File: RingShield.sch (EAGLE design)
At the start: 37 parts, among them U1 LED-ADDRESSABLE16MM, U10 LED-ADDRESSABLE16MM, U11 LED-ADDRESSABLE16MM, U12 LED-ADDRESSABLE16MM, U13 LED-ADDRESSABLE16MM, U14 LED-ADDRESSABLE16MM, U15 LED-ADDRESSABLE16MM, U16 LED-ADDRESSABLE16MM, U17 LED-ADDRESSABLE16MM, U18 LED-ADDRESSABLE16MM, U19 LED-ADDRESSABLE16MM, U2 LED-ADDRESSABLE16MM, U20 LED-ADDRESSABLE16MM, U21 LED-ADDRESSABLE16MM, U22 LED-ADDRESSABLE16MM, U23 LED-ADDRESSABLE16MM, U24 LED-ADDRESSABLE16MM, U25 LED-ADDRESSABLE16MM, U26 LED-ADDRESSABLE16MM, U27 LED-ADDRESSABLE16MM, U28 LED-ADDRESSABLE16MM, U29 LED-ADDRESSABLE16MM, U3 LED-ADDRESSABLE16MM, U30 LED-ADDRESSABLE16MM, U4 LED-ADDRESSABLE16MM, U5 LED-ADDRESSABLE16MM, U6 LED-ADDRESSABLE16MM, U7 LED-ADDRESSABLE16MM, U8 LED-ADDRESSABLE16MM, U9 LED-ADDRESSABLE16MM

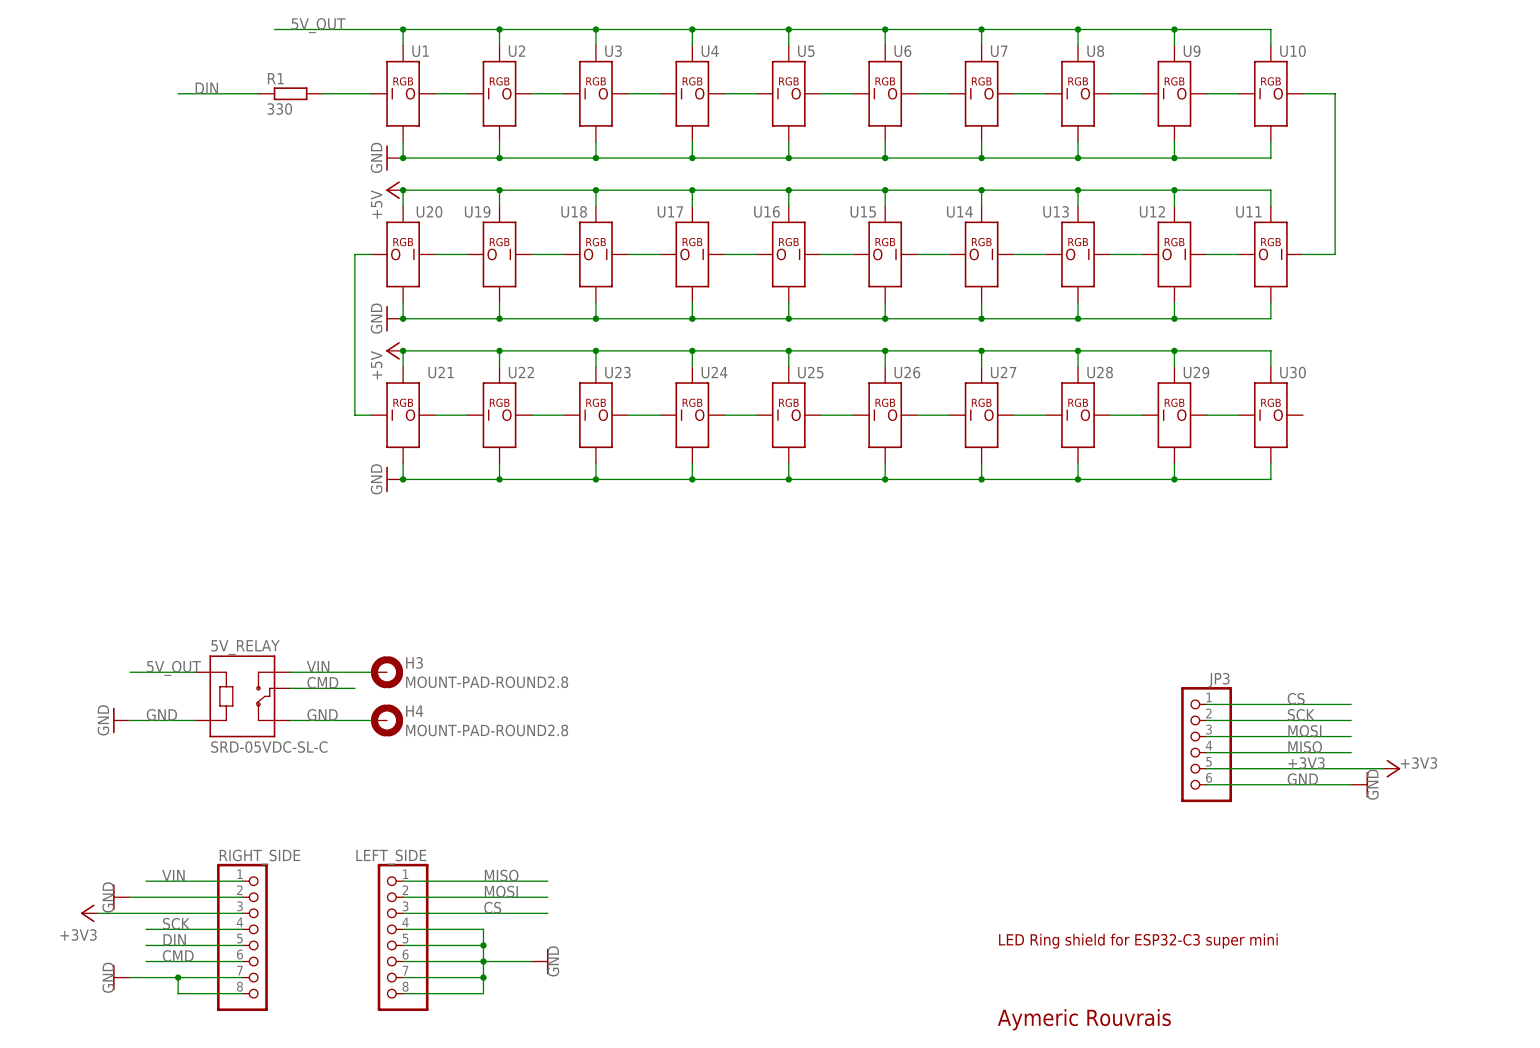
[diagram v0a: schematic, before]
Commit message: Adding v1.4
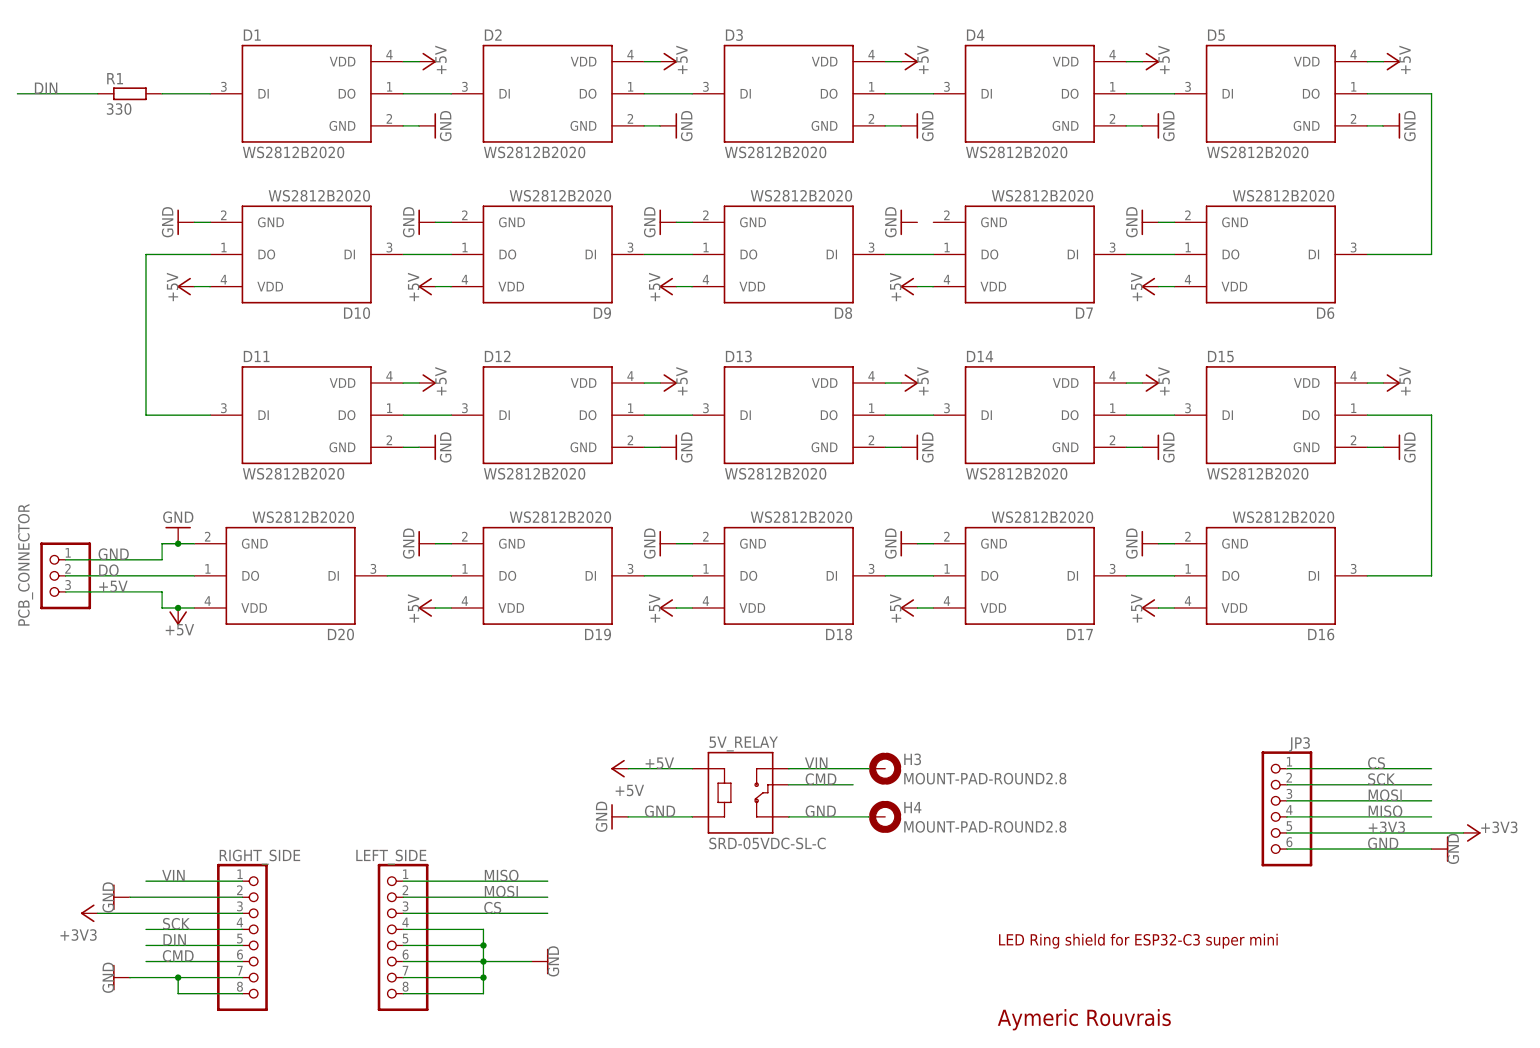
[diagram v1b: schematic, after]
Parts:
- removed U1, U10, U11, U12, U13, U14, U15, U16, U17, U18, U19, U2, U20, U21, U22, U23, U24, U25, U26, U27, U28, U29, U3, U30, U4, U5, U6, U7, U8, U9: LED-ADDRESSABLE16MM, ALBERT:LED-ADDRESSABLE16MM
- added D1, D10, D11, D12, D13, D14, D15, D16, D17, D18, D19, D2, D20, D3, D4, D5, D6, D7, D8, D9: WS2812B2020, WS2812B2020:WS2812B2020
- added PCB_CONNECTOR: (no value), pinhead:PINHD-1X3/90
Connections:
- removed net 5V_OUT: 5V_RELAY.A1, U1.VDD, U10.VDD, U2.VDD, U3.VDD, U4.VDD, U5.VDD, U6.VDD, U7.VDD, U8.VDD, U9.VDD
- removed net N$18: U12.DO, U13.DI
- removed net N$23: U20.DO, U21.DI
- removed net N$24: U21.DO, U22.DI
- removed net N$25: U22.DO, U23.DI
- removed net N$26: U23.DO, U24.DI
- removed net N$27: U24.DO, U25.DI
- removed net N$28: U25.DO, U26.DI
- removed net N$29: U26.DO, U27.DI
- removed net N$30: U27.DO, U28.DI
- removed net N$31: U28.DO, U29.DI
- removed net N$32: U29.DO, U30.DI
- new net DO: D20.DO, PCB_CONNECTOR.2
- new net N$9: D10.DI, D9.DO
- net +5V: now also 5V_RELAY.A1, D1.VDD, D10.VDD, D11.VDD, D12.VDD, D13.VDD, D14.VDD, D15.VDD, D16.VDD, D17.VDD, D18.VDD, D19.VDD, D2.VDD, D20.VDD, D3.VDD, D4.VDD, D5.VDD, D6.VDD, D7.VDD, D8.VDD, D9.VDD, PCB_CONNECTOR.3; no longer U11.VDD, U12.VDD, U13.VDD, U14.VDD, U15.VDD, U16.VDD, U17.VDD, U18.VDD, U19.VDD, U20.VDD, U21.VDD, U22.VDD, U23.VDD, U24.VDD, U25.VDD, U26.VDD, U27.VDD, U28.VDD, U29.VDD, U30.VDD
- net GND: now also D1.GND, D10.GND, D11.GND, D12.GND, D13.GND, D14.GND, D15.GND, D16.GND, D17.GND, D18.GND, D19.GND, D2.GND, D20.GND, D3.GND, D4.GND, D5.GND, D6.GND, D8.GND, D9.GND, PCB_CONNECTOR.1; no longer U1.GND, U10.GND, U11.GND, U12.GND, U13.GND, U14.GND, U15.GND, U16.GND, U17.GND, U18.GND, U19.GND, U2.GND, U20.GND, U21.GND, U22.GND, U23.GND, U24.GND, U25.GND, U26.GND, U27.GND, U28.GND, U29.GND, U3.GND, U30.GND, U4.GND, U5.GND, U6.GND, U7.GND, U8.GND, U9.GND
- net N$1: now also D1.DI, R1.2; no longer U1.DO, U2.DI
- net N$10: now also D8.DO, D9.DI; no longer U7.DO, U8.DI
- net N$11: now also D7.DO, D8.DI; no longer U8.DO, U9.DI
- net N$12: now also D6.DO, D7.DI; no longer U10.DI, U9.DO
- net N$13: now also D14.DO, D15.DI; no longer U10.DO, U11.DI
- net N$14: now also D13.DO, D14.DI; no longer U15.DO, U16.DI
- net N$15: now also D12.DO, D13.DI; no longer U16.DO, U17.DI
- net N$16: now also D11.DO, D12.DI; no longer U17.DO, U18.DI
- net N$17: now also D10.DO, D11.DI; no longer U11.DO, U12.DI
- net N$19: now also D17.DO, D18.DI; no longer U13.DO, U14.DI
- net N$2: now also D1.DO, D2.DI; no longer U2.DO, U3.DI
- net N$20: now also D16.DO, D17.DI; no longer U14.DO, U15.DI
- net N$21: now also D15.DO, D16.DI; no longer U18.DO, U19.DI
- net N$22: now also D19.DO, D20.DI; no longer U19.DO, U20.DI
- net N$3: now also D2.DO, D3.DI; no longer U3.DO, U4.DI
- net N$4: now also D3.DO, D4.DI; no longer U4.DO, U5.DI
- net N$5: now also D4.DO, D5.DI; no longer U5.DO, U6.DI
- net N$6: now also D5.DO, D6.DI; no longer U6.DO, U7.DI
- net N$7: now also D18.DO, D19.DI; no longer R1.2, U1.DI
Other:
- moved on the sheet: 5V_RELAY, H3, H4, JP3, R1
